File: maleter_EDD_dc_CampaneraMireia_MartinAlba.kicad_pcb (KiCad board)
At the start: 2 copper layers, 80.8 x 76.5 mm, 58 parts, among them J1 Conn_01x02_Pin, J2 DE9_Pins, J3 DE9_Pins, J4 Conn_01x05_Pin, M1 Motor_DC_ALT, Q1 IRLZ44N, SW1 SW_DPST_x2, SW2 SW_DPST_x2, SW3 SW_DPST_x2, SW5 SW_Push, U1 LM2596S-5, U2 LM1117DT-3.3, U3 PIC24HJ128GP502, U4 MCP2551-I-SN, U5 DRV8871DDA, U7 VL53L0CXV0DH1, U8 MAX3232, U9 LM358, Y1 8MHz

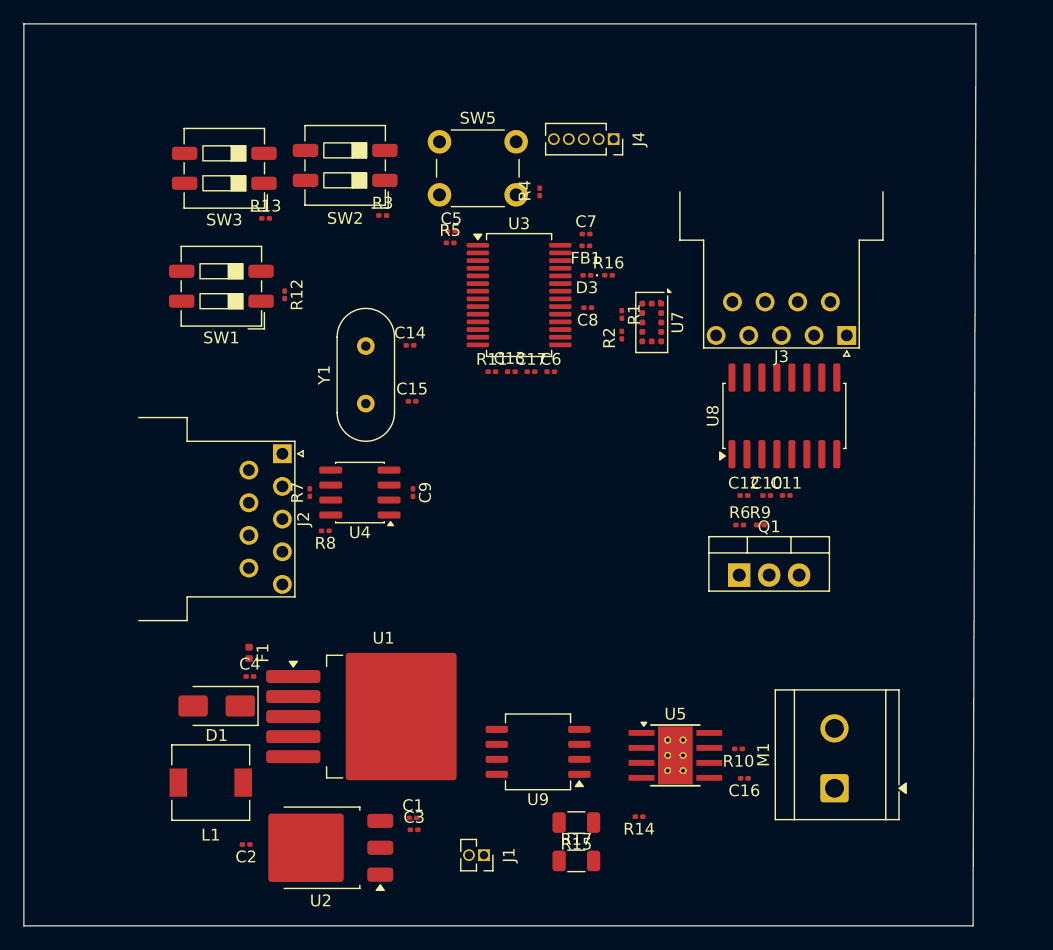
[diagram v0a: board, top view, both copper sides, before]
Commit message: lay out
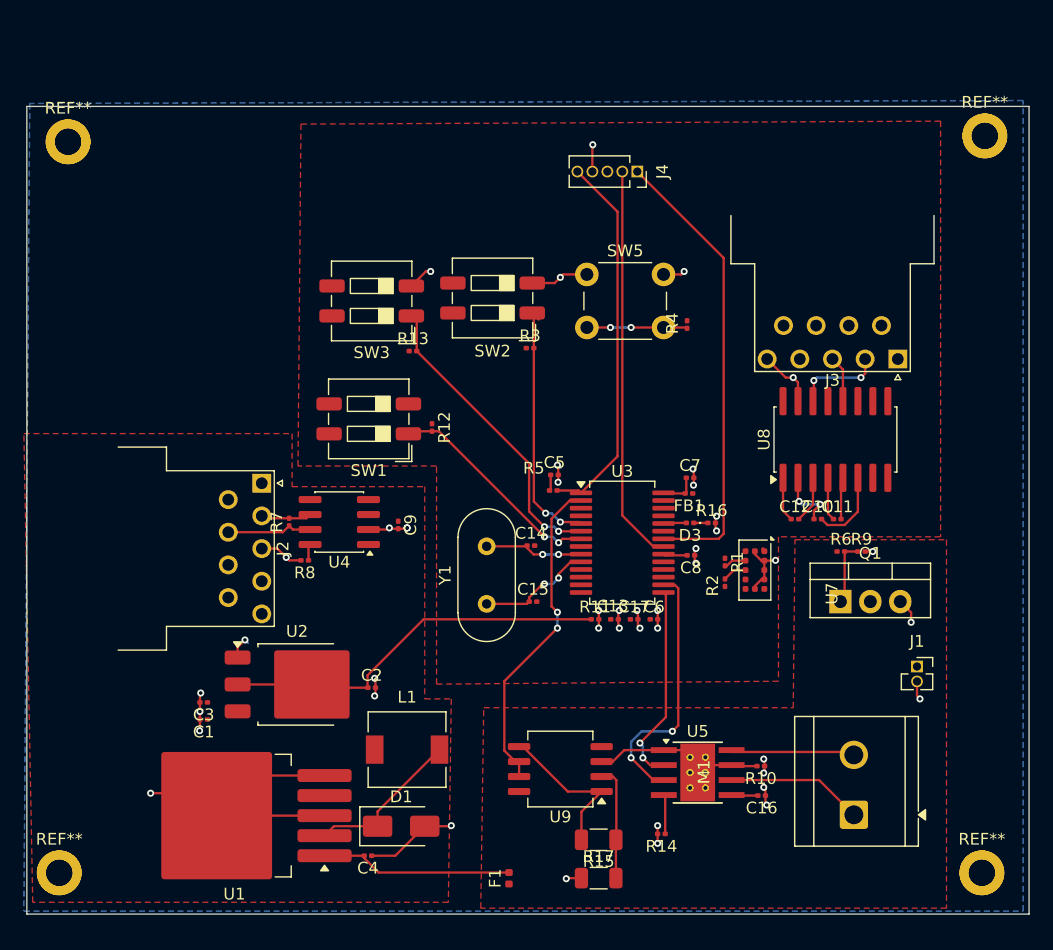
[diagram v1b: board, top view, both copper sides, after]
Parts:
- added ?: , , F.Cu at (175.8, 83.8)
- added ?: , , F.Cu at (97.2, 146.2)
- added ?: , , F.Cu at (98.0, 84.2)
- added ?: , , F.Cu at (175.5, 146.2)
- added REF**: MountingHole_2.2mm_M2_DIN965_Pad, MountingHole:MountingHole_2.2mm_M2_DIN965_Pad, F.Cu at (175.5, 146.2)
- added REF**: MountingHole_2.2mm_M2_DIN965_Pad, MountingHole:MountingHole_2.2mm_M2_DIN965_Pad, F.Cu at (175.8, 83.8)
- added REF**: MountingHole_2.2mm_M2_DIN965_Pad, MountingHole:MountingHole_2.2mm_M2_DIN965_Pad, F.Cu at (98.0, 84.2)
- added REF**: MountingHole_2.2mm_M2_DIN965_Pad, MountingHole:MountingHole_2.2mm_M2_DIN965_Pad, F.Cu at (97.2, 146.2)
- moved J1 40.1 mm to (170.0, 128.8), turned to 0 degrees
- moved F1 29.2 mm to (135.4, 146.7), turned to 90 degrees
- moved C13 22.8 mm to (144.3, 124.8)
- moved C17 22.8 mm to (146.0, 124.8)
- moved C6 22.8 mm to (147.7, 124.8)
- moved C8 22.8 mm to (150.8, 119.3)
- moved D3 22.8 mm to (150.8, 116.6)
- moved FB1 22.8 mm to (150.7, 114.1)
- moved R1 22.8 mm to (153.7, 119.9)
- moved R11 22.8 mm to (142.7, 124.8)
- moved R16 22.8 mm to (152.6, 116.6)
- moved R2 22.8 mm to (153.7, 121.6)
- moved R5 22.8 mm to (139.2, 113.8)
- moved U3 22.8 mm to (145.0, 118.2)
- moved U7 22.8 mm to (156.2, 120.6)
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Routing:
- net GND: track 0.00 -> 92.2 mm, vias 0 -> 44
- net /CONTROL UNIT/PGC: track 0.00 -> 39.0 mm
- net /CONTROL UNIT/PGD: track 0.00 -> 33.8 mm
- net 3.3V: track 0.00 -> 33.2 mm
- net MCLR: track 0.00 -> 32.1 mm
- net AntiAtrapament: track 0.00 -> 27.8 mm, vias 0 -> 2
- net Calefactor: track 0.00 -> 25.8 mm, vias 0 -> 2
- net PWM: track 0.00 -> 22.5 mm, vias 0 -> 2
- net FinalCarrera: track 0.00 -> 21.6 mm, vias 0 -> 2
- net ON/OFF: track 0.00 -> 18.8 mm, vias 0 -> 2
- net Direccio: track 0.00 -> 17.2 mm, vias 0 -> 2
- net Net-(U1-VIN): track 0.00 -> 16.3 mm
- net Net-(D1-K): track 0.00 -> 13.5 mm
- net /ALIMENTACIO I MOTOR/outamp: track 0.00 -> 13.4 mm
- net Net-(U9A-+): track 0.00 -> 12.8 mm
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- added copper zone on F.Cu, net +12V
- added copper zone on F.Cu, net +5V
- added copper zone on F.Cu, net 3.3V
- added copper zone on B.Cu, net GND
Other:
- board size 80.8 x 76.5 mm -> 85 x 68.5 mm
